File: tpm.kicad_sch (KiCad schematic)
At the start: 3 parts, among them J6 PinHeader_2x7_P2.54mm_Drill1.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

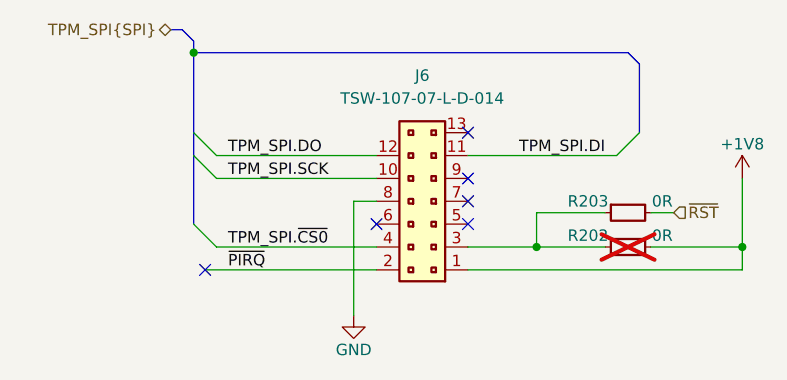
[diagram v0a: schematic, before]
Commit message: [#83609] Reannotate board
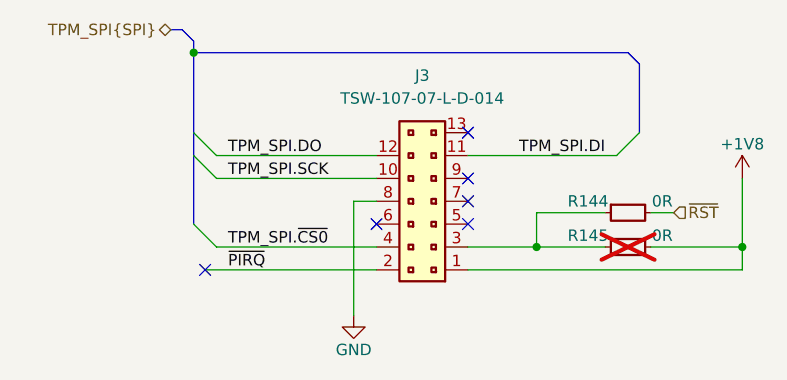
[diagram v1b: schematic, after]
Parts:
- renumbered J6 to J3, R203 to R144, R202 to R145
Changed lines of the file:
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@@
 		(dnp no)
 		(fields_autoplaced yes)
-		(property "Reference" "J6"
+		(property "Reference" "J3"
 			(at 212.09 129.54 0)
 			(effects
@@
 			(project ""
 				(path "/5f636c45-3c15-4731-8931-4625e0dab7e4/757bd70a-5179-4368-9172-3adb38876975"
-					(reference "J6")
+					(reference "J3")
 					(unit 1)
 				)
@@
 		(on_board yes)
 		(dnp no)
-		(property "Reference" "R203"
+		(property "Reference" "R144"
 			(at 230.505 143.51 0)
 			(effects
@@
 			(project "bmc-reference-carrier-board"
 				(path "/5f636c45-3c15-4731-8931-4625e0dab7e4/757bd70a-5179-4368-9172-3adb38876975"
-					(reference "R203")
+					(reference "R144")
 					(unit 1)
 				)
@@
 		(on_board yes)
 		(dnp no)
-		(property "Reference" "#PWR0289"
+		(property "Reference" "#PWR0103"
 			(at 262.89 143.51 0)
 			(effects
@@
 			(project "bmc-reference-carrier-board"
 				(path "/5f636c45-3c15-4731-8931-4625e0dab7e4/757bd70a-5179-4368-9172-3adb38876975"
-					(reference "#PWR0289")
+					(reference "#PWR0103")
 					(unit 1)
 				)
@@
 		(on_board yes)
 		(dnp no)
-		(property "Reference" "#PWR0261"
+		(property "Reference" "#PWR0102"
 			(at 213.36 158.75 0)
 			(effects
@@
 			(project ""
 				(path "/5f636c45-3c15-4731-8931-4625e0dab7e4/757bd70a-5179-4368-9172-3adb38876975"
-					(reference "#PWR0261")
+					(reference "#PWR0102")
 					(unit 1)
 				)
@@
 		(on_board yes)
 		(dnp yes)
-		(property "Reference" "R202"
+		(property "Reference" "R145"
 			(at 230.505 147.32 0)
 			(effects
@@
 			(project ""
 				(path "/5f636c45-3c15-4731-8931-4625e0dab7e4/757bd70a-5179-4368-9172-3adb38876975"
-					(reference "R202")
+					(reference "R145")
 					(unit 1)
 				)
